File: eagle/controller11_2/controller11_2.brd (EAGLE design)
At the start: 30 x 65 mm, 62 parts, among them IC1 ILD213T, IC2 MCP170312MB, J3 CONN_20X2, J5 CORTEX_DEBUG_PTH, Q2 200mA/50V, SW1 KSS221GLFS, U2 ATSAMD21G-A, U3 MP2307, X1 1501_04, X2 ZX62D-B-5PA8, Y2 32.768kHz

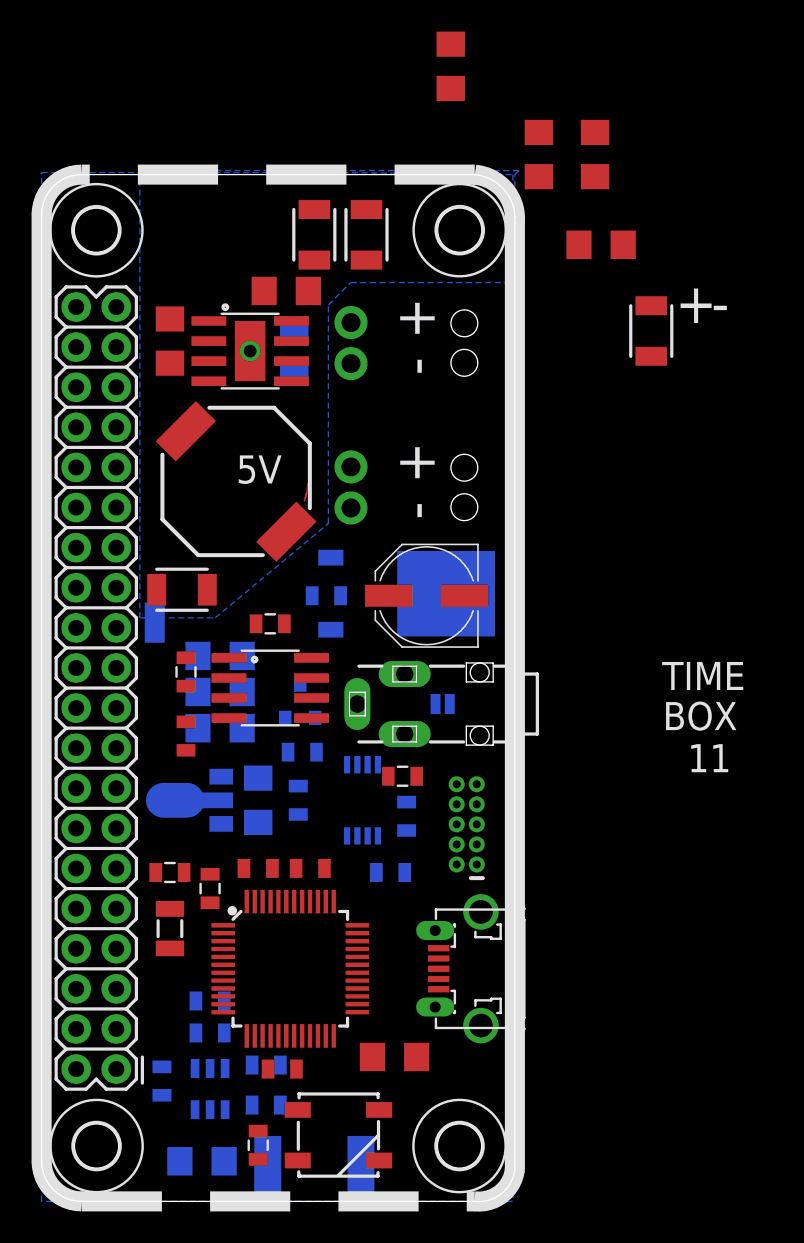
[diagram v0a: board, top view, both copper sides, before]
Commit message: progress controller11_2
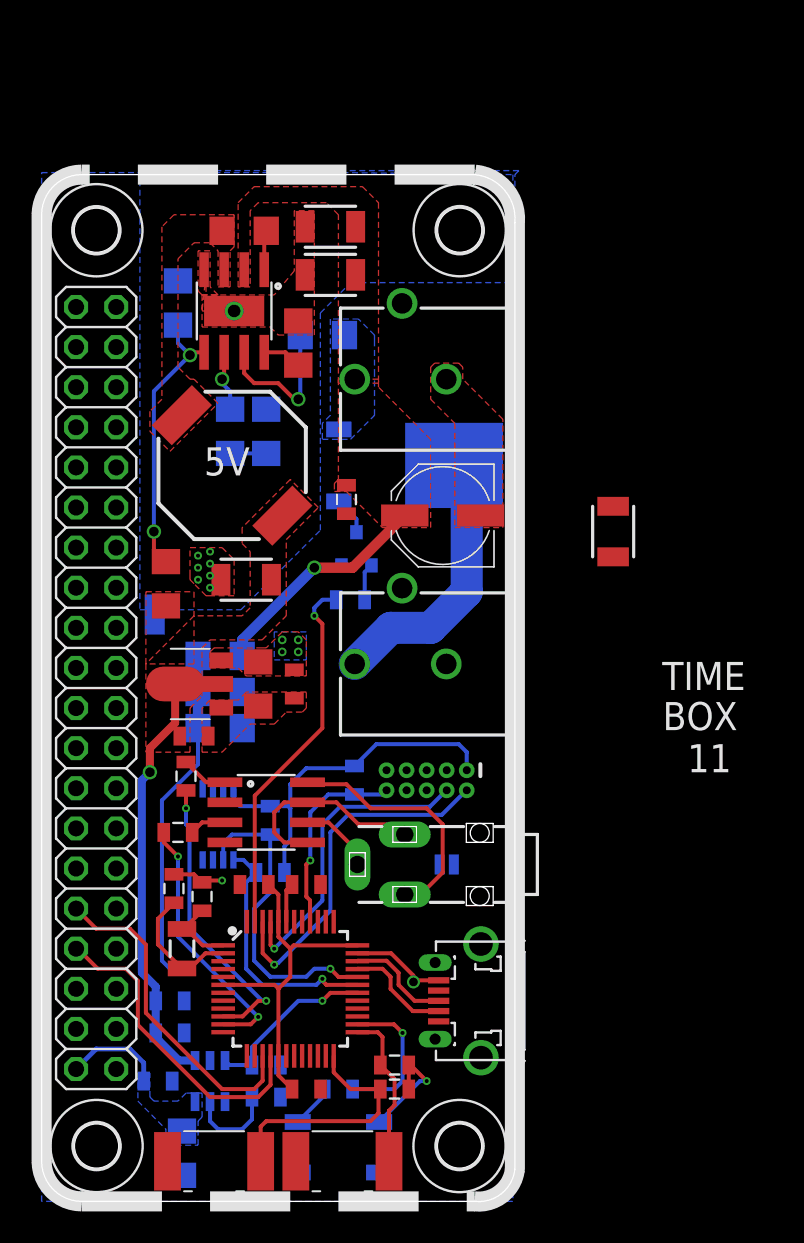
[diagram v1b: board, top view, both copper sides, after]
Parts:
- removed J3: CONN_20X2, SparkFun-Connectors:2X20
- removed U$4, U$5: NANOFIT2, volzolib:NANOFIT2
- added J1, J2: POWER_JACKPTH_BREAD, SparkFun-Connectors:POWER_JACK_PTH_BREAD
- added JP2: (no value), adafruit:2X20
- added RBTN1: 10k, SparkFun-Passives:0805
- added SW2: KSS221GLFS, adafruit:BTN_CK_KSS
- R_LED: device SparkFun-Resistors:1206 -> SparkFun-Resistors:0805
- moved R3 38.4 mm to (7.87, 39.1), turned to 270 degrees
- moved C17 30.1 mm to (13.0, 39.4), turned to 0 degrees
- moved C16 27.6 mm to (36.2, 42.4), turned to 270 degrees
- moved R2 27.0 mm to (8.64, 56.9), flipped to the bottom, turned to 90 degrees
- moved C14 26.3 mm to (11.9, 48.8), flipped to the bottom, turned to 90 degrees
- moved R1 25.9 mm to (14.2, 48.8), flipped to the bottom, turned to 90 degrees
- moved R20 11.0 mm to (9.14, 26.9), turned to 90 degrees
- moved Q2 10.3 mm to (19.9, 41.3)
- moved R15 10.2 mm to (8.64, 23.4), turned to 0 degrees
- moved JP1 10.2 mm to (25.7, 21.3)
- moved X1 10.2 mm to (31.5, 21.3)
- moved R10 10.1 mm to (19.6, 38.1)
- moved RBTN 9.34 mm to (22.4, 7.11), turned to 180 degrees
- moved MCP9808 9.27 mm to (11.2, 23.9)
- moved R_I2C_1 8.64 mm to (14.5, 24.1)
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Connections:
- net USB1_EN renamed ZERO_EN
- removed net BTN: RBTN.2, SW1.P$2, U2.25
- removed net USB1_OUT: AP2553.6, C3.2, C4.2
- removed net USB2_EN: U2.28
- removed net USB_5V: AP2553.1, C1.1, C2.1, C7.1, IC2.2@1
- new net BTN1: RBTN.2, SW1.P$2, U2.24
- new net BTN2: RBTN1.2, SW2.P$2, U2.25
- net BATT_VCC: now also J1.PWR; no longer U$4.P$2
- net CAM1: now also U2.10
- net CAM2: now also U2.11
- net CAM_EN: now also U2.47
- net CAM_OUT: now also J2.PWR; no longer U$5.P$2
- net CONV_5V: now also AP2553.1, C1.1, C2.1, C7.1, IC2.2@1
- net GND: now also J1.GND, J2.GND, JP2.6, SW2.P$1; no longer J3.6, U$4.P$1, U$5.P$1
- net VCC: now also RBTN1.1
- net VD_DIRECT: now also U2.7
- net ZERO_5V: now also AP2553.6, C3.2, C4.2, JP2.2; no longer J3.2
- net ZERO_RX: now also JP2.10, U2.15; no longer J3.10
- net ZERO_TX: now also JP2.8, U2.16; no longer J3.8
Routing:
- net VCC: track 0.00 -> 53.8 mm, vias 0 -> 5
- net CONV_5V: track 0.00 -> 26.7 mm, vias 0 -> 1
- net CAM_EN: track 0.00 -> 23.5 mm, vias 0 -> 1
- net SWDIO: track 0.00 -> 22.7 mm, vias 0 -> 1
- net VD_DIRECT: track 0.00 -> 21.5 mm
- net ZERO_RX: track 0.00 -> 21.2 mm
- net SCL: track 0.00 -> 20.2 mm, vias 0 -> 1
- net ZERO_TX: track 0.00 -> 20.0 mm
- net SWDCLK: track 0.00 -> 19.7 mm, vias 0 -> 1
- net CAM1: track 0.00 -> 18.7 mm, vias 0 -> 2
- net N$30: track 0.00 -> 17.5 mm, vias 0 -> 2
- net CAM2: track 0.00 -> 16.6 mm, vias 0 -> 2
- net CAM_OUT: track 0.00 -> 16.1 mm
- net SDA: track 0.00 -> 16.0 mm, vias 0 -> 1
- net BTN1: track 0.00 -> 16.0 mm
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- added copper zone on layer 1, net BATT_VCC
- added copper zone on layer 16, net BATT_VCC
- added copper zone on layer 1, net GND
- added copper zone on layer 1, net GNDA
- added copper zone on layer 1, net N$26
- added copper zone on layer 1, net VCC
- added copper zone on layer 16, net VCC
- added copper zone on layer 16, net ZERO_5V
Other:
- board text removed: "+"
- board text removed: "-"
